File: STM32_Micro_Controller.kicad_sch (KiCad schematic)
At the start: 1 part, among them U1 STM32F103C8T6

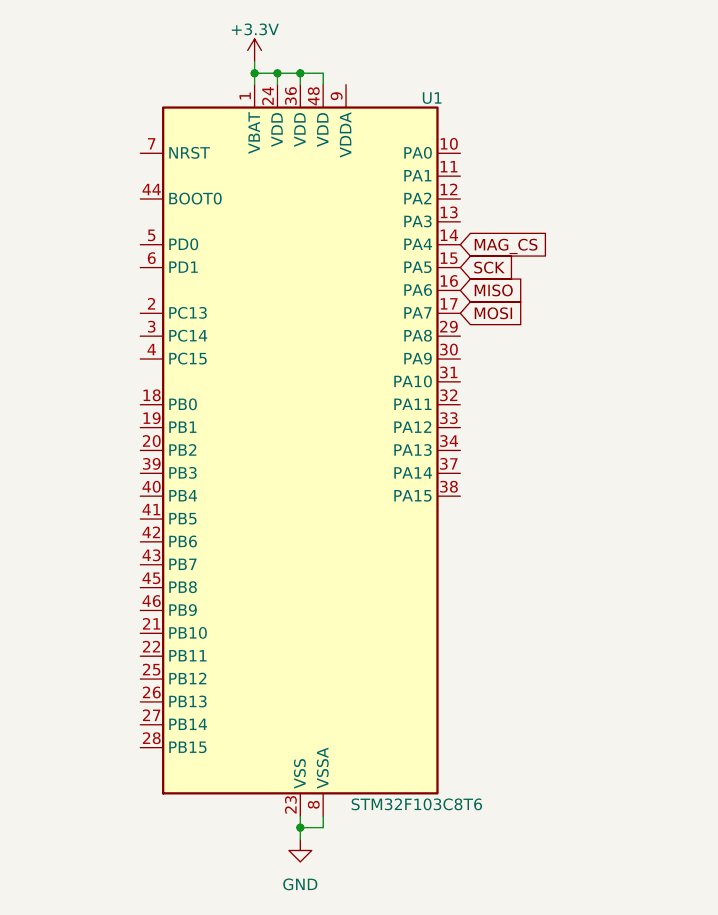
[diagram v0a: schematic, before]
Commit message: Add files via upload
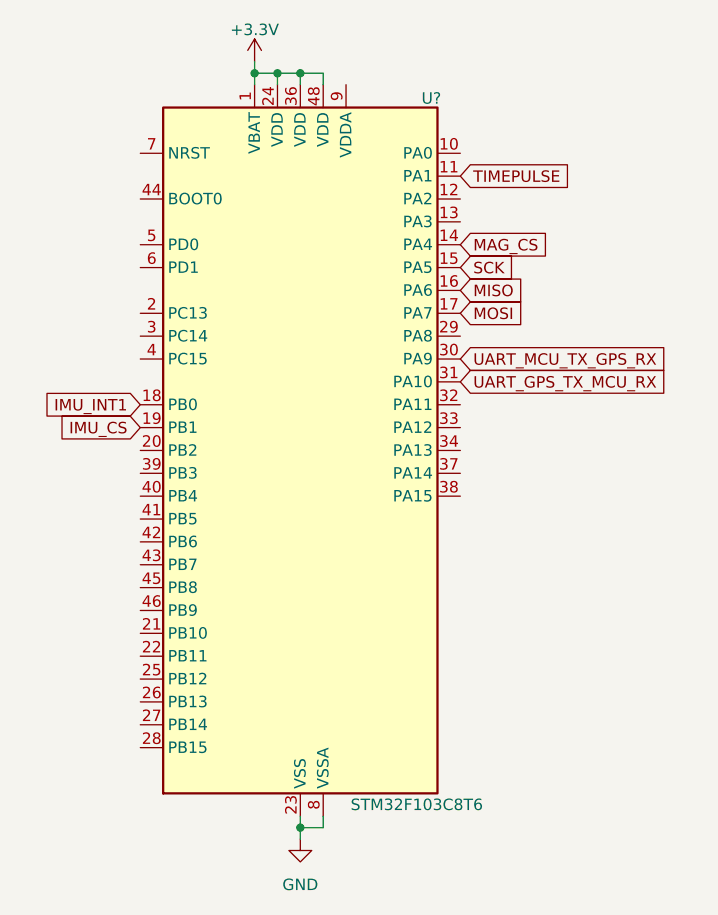
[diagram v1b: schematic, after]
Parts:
- renumbered U1 to U?
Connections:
- net TIMEPULSE: now reaches U?.11 (PA1)
- net IMU_INT1: now reaches U?.18 (PB0)
- net IMU_CS: now reaches U?.19 (PB1)
- net UART_MCU_TX_GPS_RX: now reaches U?.30 (PA9)
- net UART_GPS_TX_MCU_RX: now reaches U?.31 (PA10)
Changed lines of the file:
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@@
+		)
+	)
+	(global_label "TIMEPULSE"
+		(shape input)
+		(at 148.59 62.23 0)
+		(fields_autoplaced yes)
+		(effects
+			(font
+				(size 1.27 1.27)
+			)
+			(justify left)
+		)
+		(property "Intersheetrefs" "${INTERSHEET_REFS}"
+			(at 161.7351 62.23 0)
+			(effects
+				(font
+					(size 1.27 1.27)
+				)
+				(justify left)
+				(hide yes)
+			)
+		)
+	)
+	(global_label "IMU_INT1"
+		(shape input)
+		(at 113.03 87.63 180)
+		(fields_autoplaced yes)
+		(effects
+			(font
+				(size 1.27 1.27)
+			)
+			(justify right)
+		)
+		(property "Intersheetrefs" "${INTERSHEET_REFS}"
+			(at 101.5781 87.63 0)
+			(effects
+				(font
+					(size 1.27 1.27)
+				)
+				(justify right)
+				(hide yes)
+			)
+		)
+	)
+	(global_label "UART_MCU_TX_GPS_RX"
+		(shape input)
+		(at 148.59 82.55 0)
+		(fields_autoplaced yes)
+		(effects
+			(font
+				(size 1.27 1.27)
+			)
+			(justify left)
+		)
+		(property "Intersheetrefs" "${INTERSHEET_REFS}"
+			(at 172.5603 82.55 0)
+			(effects
+				(font
+					(size 1.27 1.27)
+				)
+				(justify left)
+				(hide yes)
+			)
 		)
 	)
@@
 				)
 				(justify left)
+				(hide yes)
+			)
+		)
+	)
+	(global_label "UART_GPS_TX_MCU_RX"
+		(shape input)
+		(at 148.59 85.09 0)
+		(fields_autoplaced yes)
+		(effects
+			(font
+				(size 1.27 1.27)
+			)
+			(justify left)
+		)
+		(property "Intersheetrefs" "${INTERSHEET_REFS}"
+			(at 172.5603 85.09 0)
+			(effects
+				(font
+					(size 1.27 1.27)
+				)
+				(justify left)
+				(hide yes)
+			)
+		)
+	)
+	(global_label "IMU_CS"
+		(shape input)
+		(at 113.03 90.17 180)
+		(fields_autoplaced yes)
+		(effects
+			(font
+				(size 1.27 1.27)
+			)
+			(justify right)
+		)
+		(property "Intersheetrefs" "${INTERSHEET_REFS}"
+			(at 103.211 90.17 0)
+			(effects
+				(font
+					(size 1.27 1.27)
+				)
+				(justify right)
 				(hide yes)
 			)
@@
 		(on_board yes)
 		(dnp no)
-		(property "Reference" "U1"
+		(property "Reference" "U?"
 			(at 144.272 53.594 0)
 			(effects
@@
 		)
 		(instances
+			(project "STM32_Micro_Controller (1)"
+				(path "/21af2904-4211-4090-9120-4036a9676746"
+					(reference "U?")
+					(unit 1)
+				)
+			)
 			(project "flight-controller-basic"
 				(path "/e04fbe87-dc7c-407c-abef-b71ed1bbe06a/9ed827cc-d6ed-4e01-b191-8b39b0ab77a8"
@@
 		(dnp no)
 		(fields_autoplaced yes)
-		(property "Reference" "#PWR01"
+		(property "Reference" "#PWR?"
 			(at 130.81 142.24 0)
 			(effects
@@
 		)
 		(instances
+			(project "STM32_Micro_Controller (1)"
+				(path "/21af2904-4211-4090-9120-4036a9676746"
+					(reference "#PWR?")
+					(unit 1)
+				)
+			)
 			(project "flight-controller-basic"
 				(path "/e04fbe87-dc7c-407c-abef-b71ed1bbe06a/9ed827cc-d6ed-4e01-b191-8b39b0ab77a8"
@@
 		(on_board yes)
 		(dnp no)
-		(property "Reference" "#PWR02"
+		(property "Reference" "#PWR?"
 			(at 125.73 53.34 0)
 			(effects
@@
 		)
 		(instances
+			(project "STM32_Micro_Controller (1)"
+				(path "/21af2904-4211-4090-9120-4036a9676746"
+					(reference "#PWR?")
+					(unit 1)
+				)
+			)
 			(project "flight-controller-basic"
 				(path "/e04fbe87-dc7c-407c-abef-b71ed1bbe06a/9ed827cc-d6ed-4e01-b191-8b39b0ab77a8"
@@
 		)
 	)
+	(sheet_instances
+		(path "/"
+			(page "1")
+		)
+	)
+	(embedded_fonts no)
 )
